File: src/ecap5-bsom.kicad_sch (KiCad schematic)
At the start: 0 parts

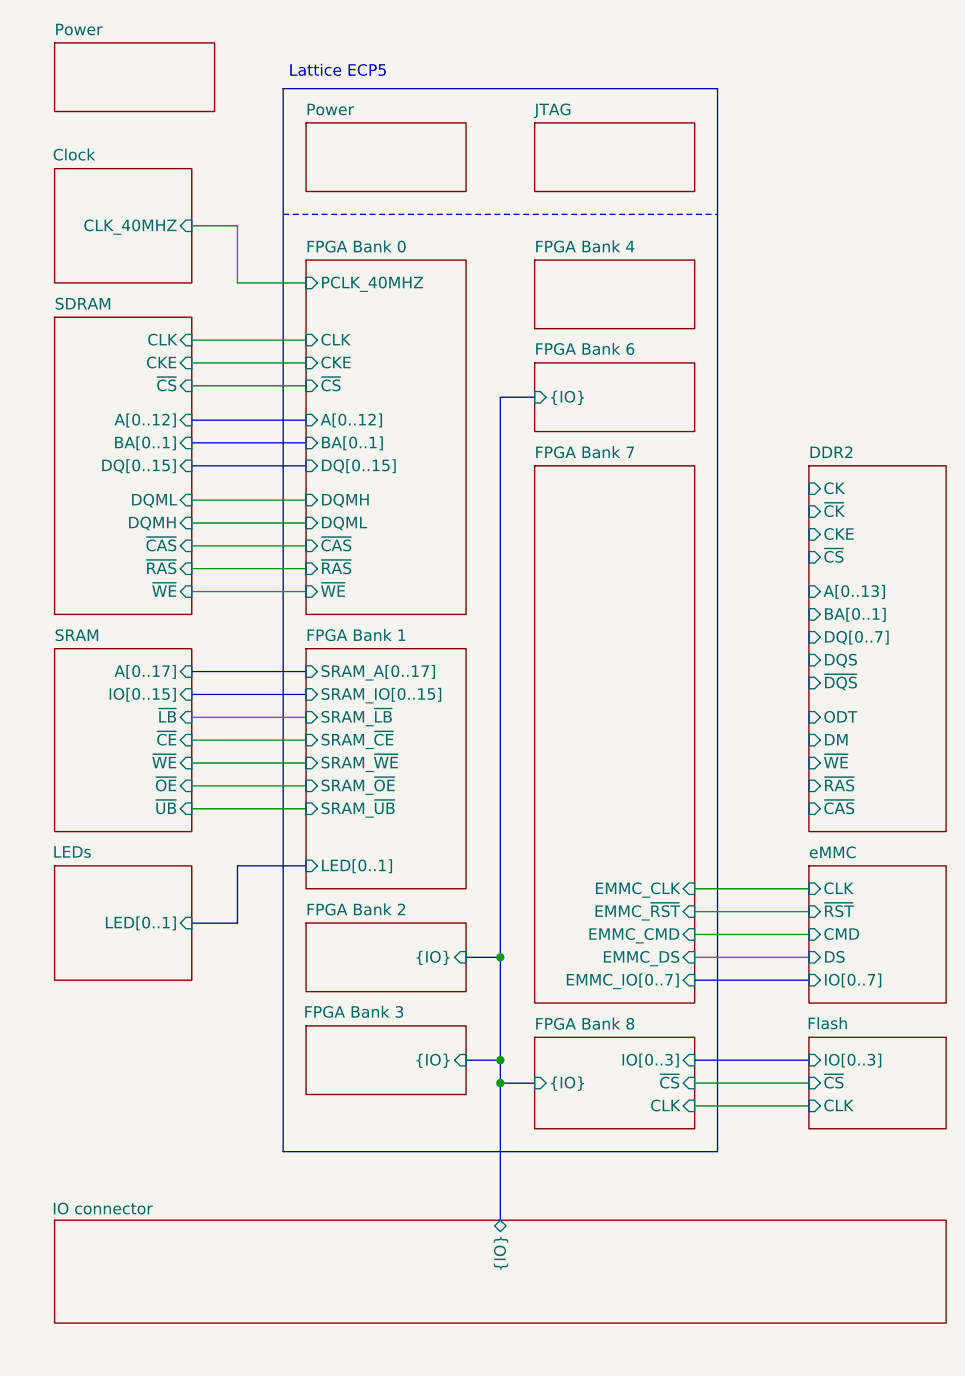
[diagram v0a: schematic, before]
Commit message: Finishes the root page
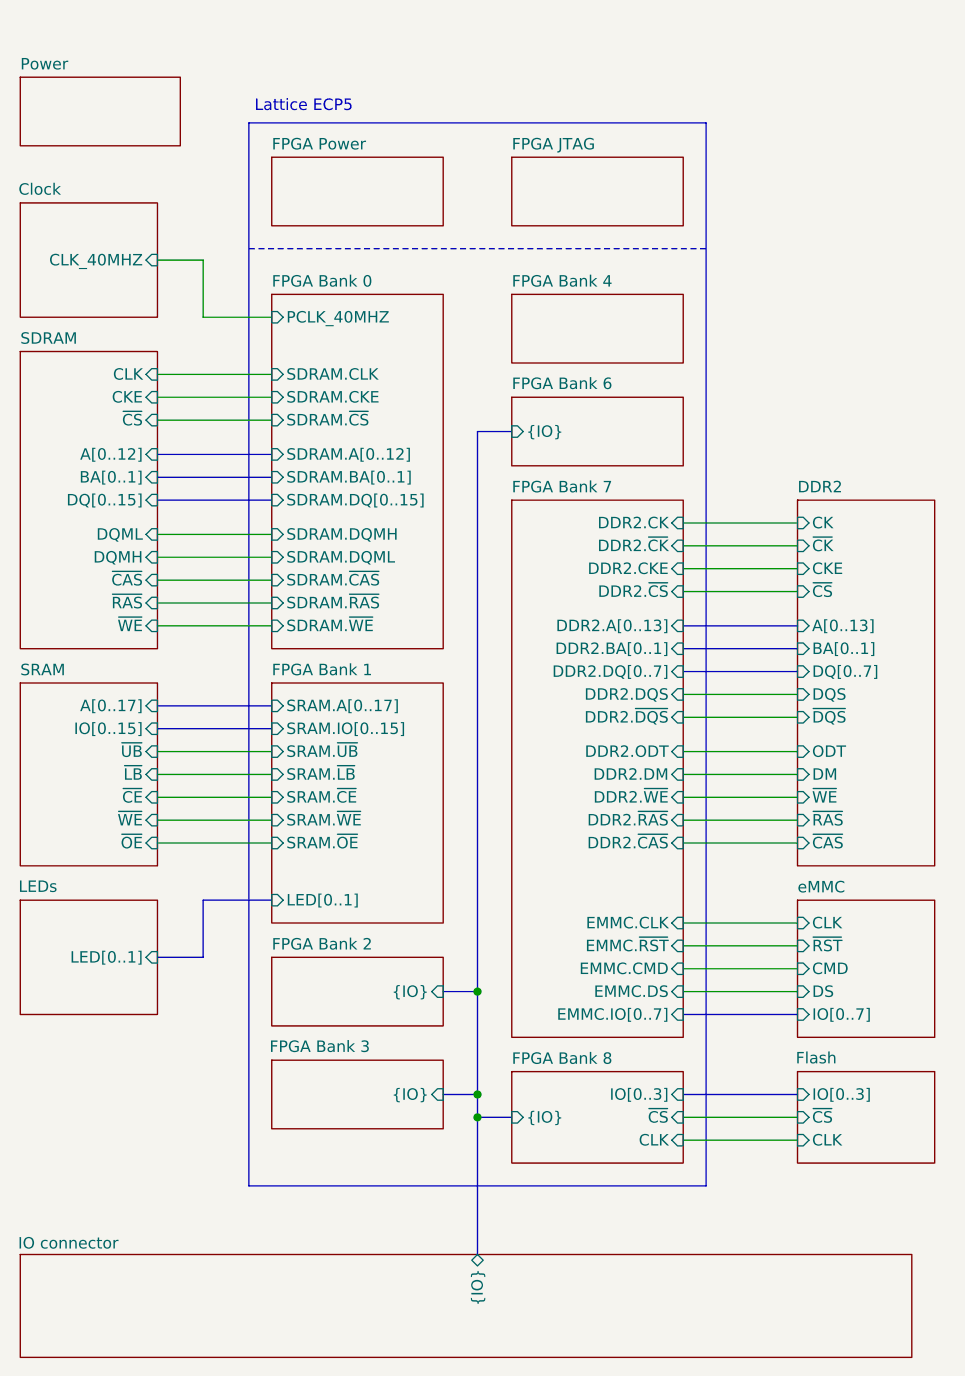
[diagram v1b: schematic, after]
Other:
- sheet JTAG renamed FPGA JTAG
- added sheet FPGA Power (schematics/fpga-power.kicad_sch)
- sheet FPGA Bank 0: file fpga-bank0.kicad_sch -> schematics/fpga-bank0.kicad_sch
- sheet FPGA Bank 0 ports: added SDRAM.A[0..12], SDRAM.BA[0..1], SDRAM.CKE, SDRAM.CLK, SDRAM.DQMH, SDRAM.DQML, SDRAM.DQ[0..15], SDRAM.~{CAS}, SDRAM.~{CS}, SDRAM.~{RAS}, SDRAM.~{WE}; removed A[0..12], BA[0..1], CKE, CLK, DQMH, DQML, DQ[0..15], ~{CAS}, ~{CS}, ~{RAS}, ~{WE}
- sheet FPGA Bank 1: file fpga-bank1.kicad_sch -> schematics/fpga-bank1.kicad_sch
- sheet FPGA Bank 1 ports: added SRAM.A[0..17], SRAM.IO[0..15], SRAM.~{CE}, SRAM.~{LB}, SRAM.~{OE}, SRAM.~{UB}, SRAM.~{WE}; removed SRAM_A[0..17], SRAM_IO[0..15], SRAM_~{CE}, SRAM_~{LB}, SRAM_~{OE}, SRAM_~{UB}, SRAM_~{WE}
- sheet FPGA Bank 2: file fpga-bank2.kicad_sch -> schematics/fpga-bank2.kicad_sch
- sheet FPGA Bank 3: file fpga-bank3.kicad_sch -> schematics/fpga-bank3.kicad_sch
- sheet FPGA Bank 4: file fpga-bank4.kicad_sch -> schematics/fpga-bank4.kicad_sch
- sheet FPGA Bank 6: file fpga-bank6.kicad_sch -> schematics/fpga-bank6.kicad_sch
- sheet FPGA Bank 7: file fpga-bank7.kicad_sch -> schematics/fpga-bank7.kicad_sch
- sheet FPGA Bank 7 ports: added DDR2.A[0..13], DDR2.BA[0..1], DDR2.CK, DDR2.CKE, DDR2.DM, DDR2.DQS, DDR2.DQ[0..7], DDR2.ODT, DDR2.~{CAS}, DDR2.~{CK}, DDR2.~{CS}, DDR2.~{DQS}, DDR2.~{RAS}, DDR2.~{WE}, EMMC.CLK, EMMC.CMD, EMMC.DS, EMMC.IO[0..7], EMMC.~{RST}; removed EMMC_CLK, EMMC_CMD, EMMC_DS, EMMC_IO[0..7], EMMC_~{RST}
- sheet FPGA Bank 8: file fpga-bank8.kicad_sch -> schematics/fpga-bank8.kicad_sch
- sheet Power: file schematics/fpga-power.kicad_sch -> schematics/power.kicad_sch
